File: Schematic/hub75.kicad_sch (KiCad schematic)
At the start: 3 parts, among them J1 Conn_02x08_Odd_Even, J3 Conn_01x04_Pin, U1 74LS08

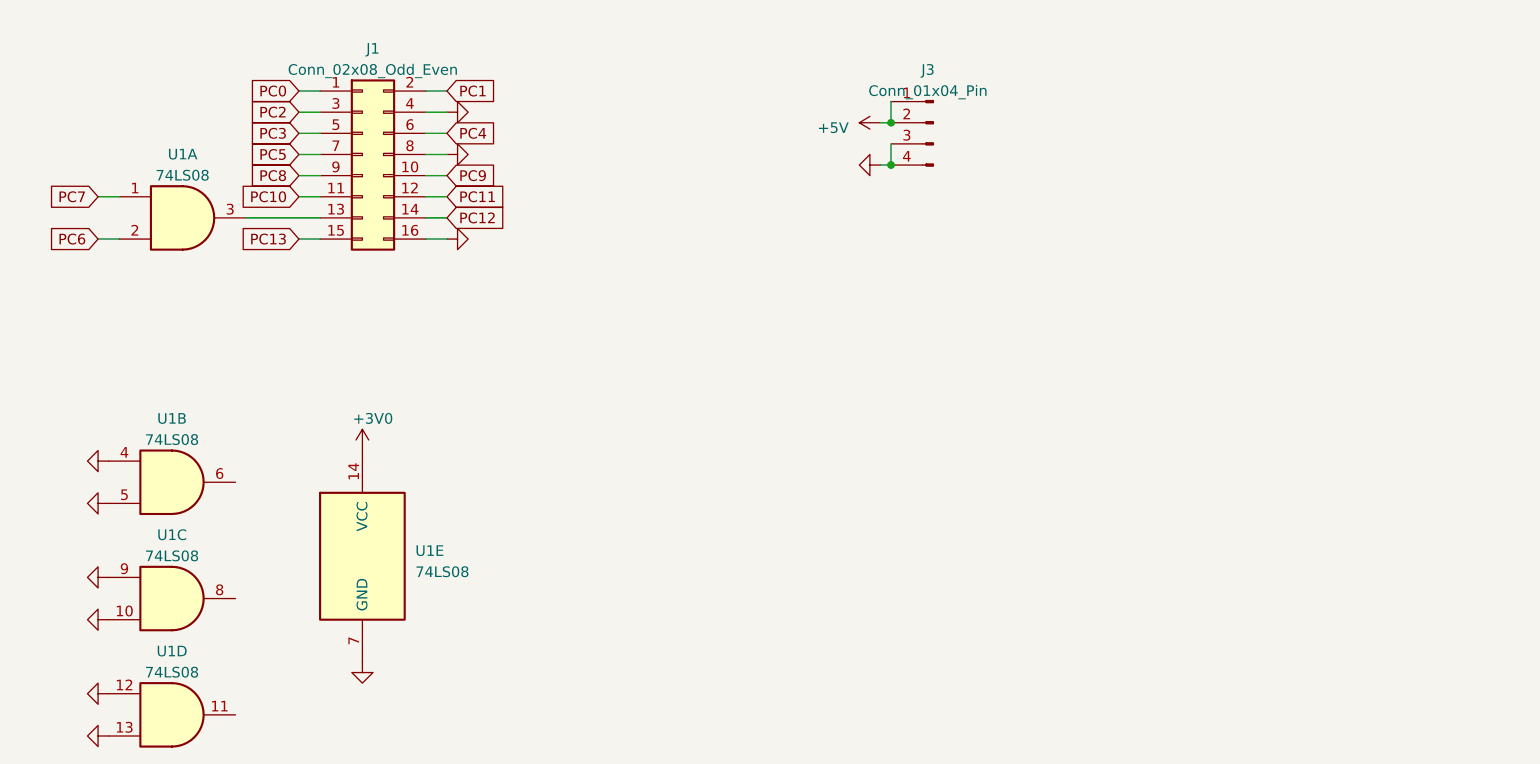
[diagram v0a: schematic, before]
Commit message: initial CB design
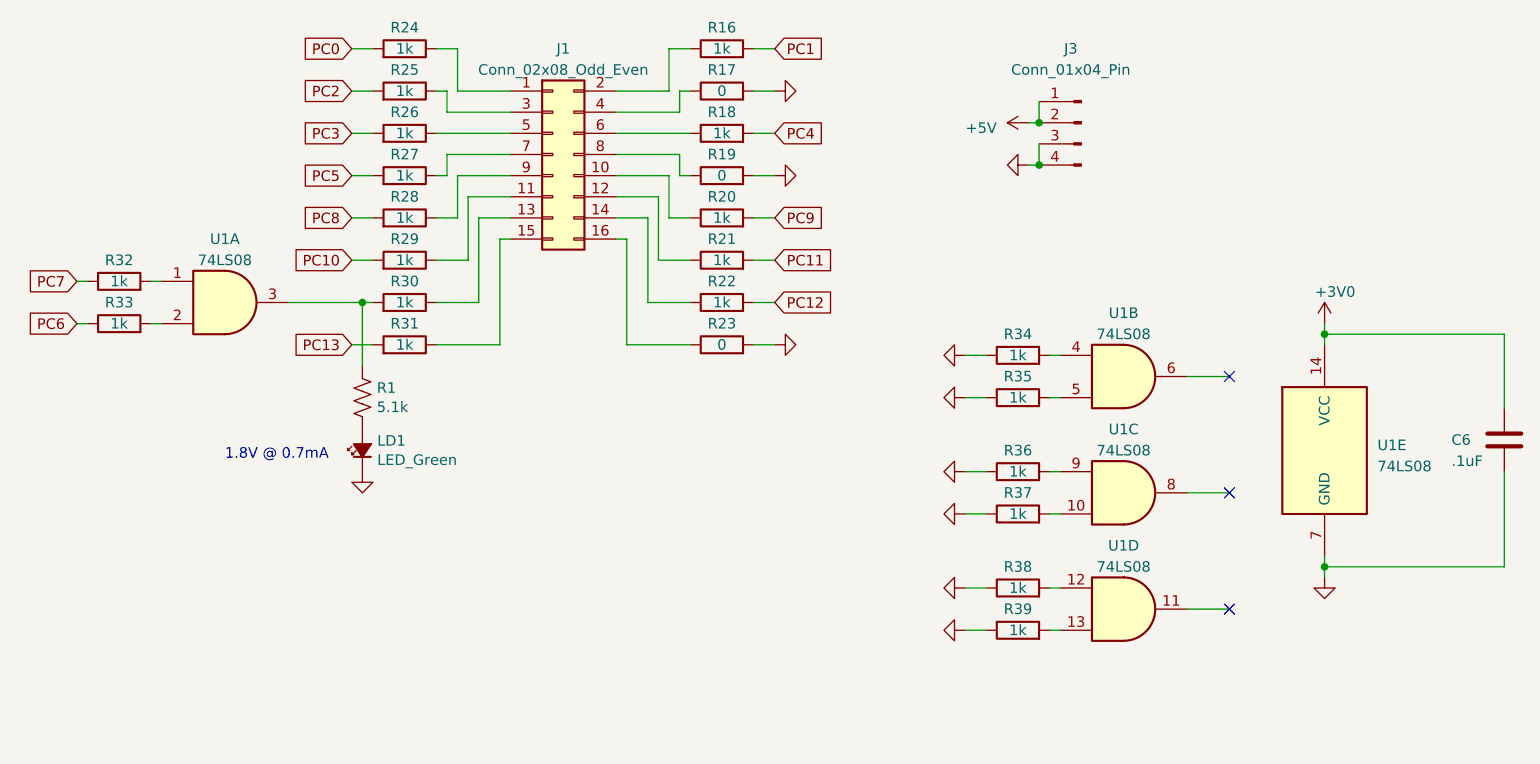
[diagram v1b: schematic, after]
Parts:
- added C6: .1uF, Capacitor_SMD:C_0805_2012Metric_Pad1.18x1.45mm_HandSolder, symbol Device:C
- added LD1: LED_Green, LED_THT:LED_D5.0mm, symbol stm32f091-rescue:LED_Small_ALT-Device
- added R1: 5.1k, Resistor_SMD:R_1206_3216Metric_Pad1.30x1.75mm_HandSolder, symbol Device:R_US
- added R16, R18, R20, R21, R22, R24, R25, R26, R27, R28, R29, R30, R31, R32, R33, R34, R35, R36, R37, R38, R39: 1k, Resistor_SMD:R_1206_3216Metric_Pad1.30x1.75mm_HandSolder, symbol Device:R
- added R17, R19, R23: 0, Resistor_SMD:R_1206_3216Metric_Pad1.30x1.75mm_HandSolder, symbol Device:R
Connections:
- net +3V0: now also C6.1
- net GND: now also C6.2, LD1.1 (K), R17.2, R19.2, R23.2, R34.1, R35.1, R36.1, R37.1, R38.1, R39.1; no longer J1.16 (Pin_16), J1.4 (Pin_4), J1.8 (Pin_8), U1.10, U1.12, U1.13, U1.4, U1.5, U1.9
- net PC0: now also R24.2; no longer J1.1 (Pin_1)
- net PC1: now also R16.2; no longer J1.2 (Pin_2)
- net PC10: now also R29.2; no longer J1.11 (Pin_11)
- net PC11: now also R21.2; no longer J1.12 (Pin_12)
- net PC12: now also R22.2; no longer J1.14 (Pin_14)
- net PC13: now also R31.2; no longer J1.15 (Pin_15)
- net PC2: now also R25.2; no longer J1.3 (Pin_3)
- net PC3: now also R26.2; no longer J1.5 (Pin_5)
- net PC4: now also R18.2; no longer J1.6 (Pin_6)
- net PC5: now also R27.2; no longer J1.7 (Pin_7)
- net PC6: now also R33.1; no longer U1.2
- net PC7: now also R32.1; no longer U1.1
- net PC8: now also R28.2; no longer J1.9 (Pin_9)
- net PC9: now also R20.2; no longer J1.10 (Pin_10)
- net at J1.13 (Pin_13): now also R30.1; no longer U1.3
- new net: R37.2, U1.10
- new net: R36.2, U1.9
- new net: J1.15 (Pin_15), R31.1
- new net: R32.2, U1.1
- new net: J1.3 (Pin_3), R25.1
- new net: J1.6 (Pin_6), R18.1
- new net: J1.16 (Pin_16), R23.1
- new net: R1.1, R30.2, U1.3
- new net: R38.2, U1.12
- new net: R33.2, U1.2
- new net: LD1.2 (A), R1.2
- new net: J1.7 (Pin_7), R27.1
- new net: R34.2, U1.4
- new net: R35.2, U1.5
- new net: J1.14 (Pin_14), R22.1
- new net: J1.2 (Pin_2), R16.1
- new net: R39.2, U1.13
- new net: J1.11 (Pin_11), R29.1
- new net: J1.9 (Pin_9), R28.1
- new net: J1.12 (Pin_12), R21.1
- new net: J1.1 (Pin_1), R24.1
- new net: J1.10 (Pin_10), R20.1
- new net: J1.4 (Pin_4), R17.1
- new net: J1.5 (Pin_5), R26.1
- new net: J1.8 (Pin_8), R19.1
- no-connect marks 0 -> 3
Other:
- note added: "1.8V @ 0.7mA"
- moved on the sheet: J1, J3, U1A, U1B, U1C, U1D, U1E
